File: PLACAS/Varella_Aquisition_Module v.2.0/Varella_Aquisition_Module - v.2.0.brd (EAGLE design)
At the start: 100 x 80 mm, 70 parts, among them IC1 M95M04-DRDW6TP, IC10 ICL7660SCBAZ, IC3 M95M04-DRDW6TP, IC4 M95M04-DRDW6TP, IC9 M95M04-DRDW6TP, U1 FT232RLSSOP, X2 USB-SMD-NS, Y2 FA-20H_16.0000MF10Z-AJ0

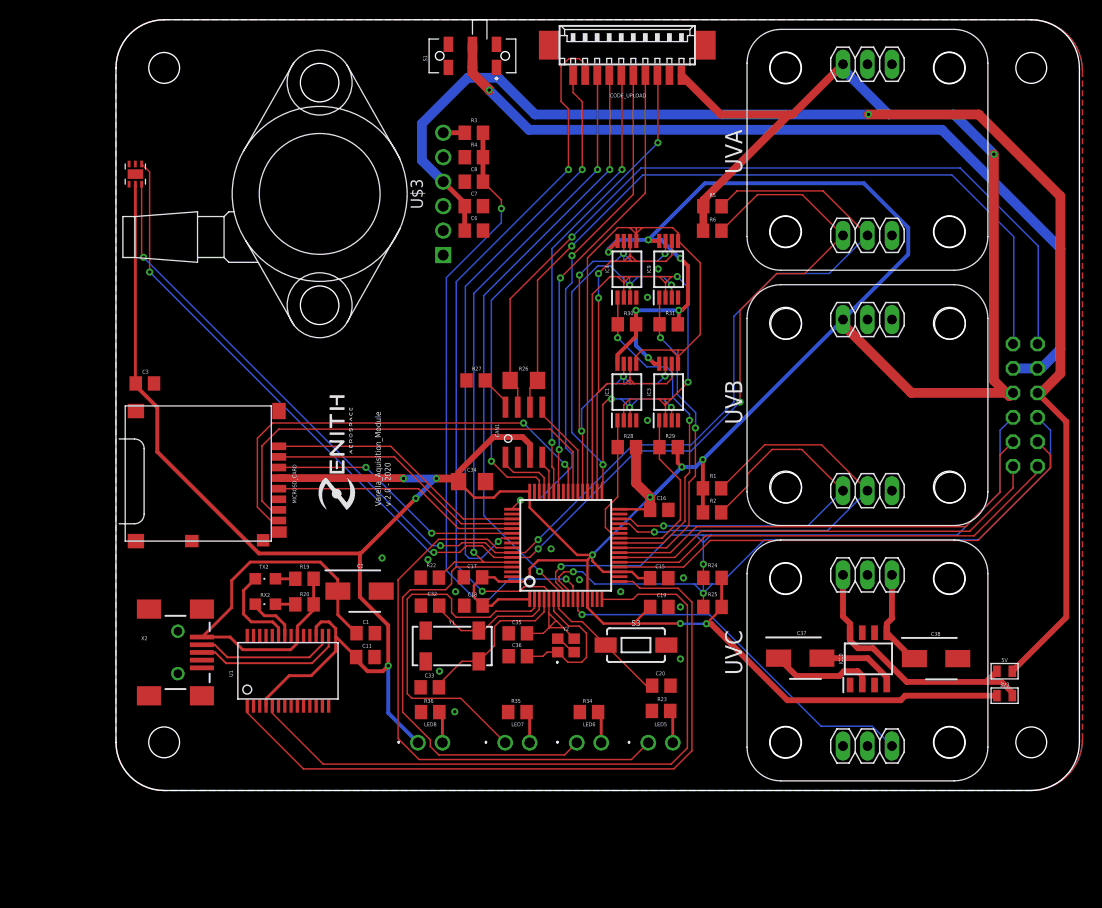
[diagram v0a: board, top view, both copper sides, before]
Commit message: Add files via upload
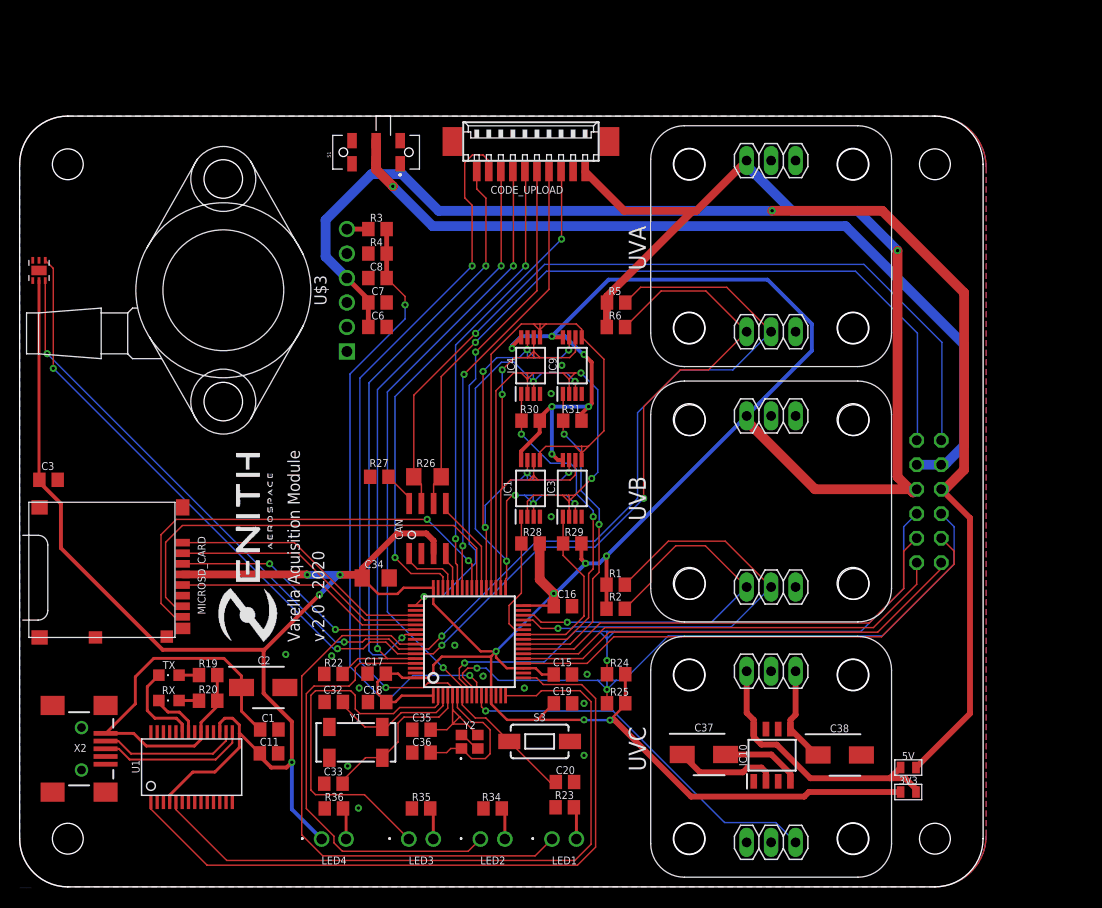
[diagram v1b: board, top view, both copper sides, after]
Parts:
- removed CAN1: SN65HVD233D, SN65HVD233D:SOIC8
- removed LED5, LED6, LED7, LED8: TLLG4400-AS12, SamacSys_Parts:TLLG4400AS12
- removed RX2, TX2: (no value), led:CHIPLED_0805
- added CAN: SN65HVD233D, SN65HVD233D:SOIC8
- added LED1, LED2, LED3, LED4: TLLG4400-AS12, SamacSys_Parts:TLLG4400AS12
- added RX, TX: (no value), led:CHIPLED_0805
- moved C20 14.1 mm to (56.6, 10.9)
- moved COMM_MICRO2 14.1 mm to (46.7, 25.4)
- moved IC3 14.1 mm to (57.4, 41.4)
- moved R29 14.1 mm to (57.4, 35.6)
- moved R6 14.1 mm to (61.9, 58.1)
- moved U$2 14.1 mm to (2.01, 64.0)
- moved U$3 14.1 mm to (34.0, 55.6)
- moved 3V3 14.1 mm to (92.2, 9.84)
- moved 5V 14.1 mm to (92.2, 12.4)
- moved C11 14.1 mm to (25.9, 13.9)
- moved C18 14.1 mm to (37.1, 19.2)
- moved C2 14.1 mm to (25.3, 20.7)
- moved C3 14.1 mm to (3.00, 42.2)
- moved C32 14.1 mm to (32.6, 19.2)
- moved C33 14.1 mm to (32.6, 10.7)
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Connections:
- net +3V3: now also CAN.3, LED4.1; no longer CAN1.3, LED8.1
- net CAN1_LBK: now also CAN.5; no longer CAN1.5
- net CAN1_RX: now also CAN.4; no longer CAN1.4
- net CAN1_TX: now also CAN.1; no longer CAN1.1
- net CAN_H: now also CAN.7; no longer CAN1.7
- net CAN_L: now also CAN.6; no longer CAN1.6
- net GND: now also CAN.2; no longer CAN1.2
- net LED_DEBUG: now also LED3.1; no longer LED7.1
- net LED_SD: now also LED1.1; no longer LED5.1
- net LED_USB: now also LED2.1; no longer LED6.1
- net N$11: now also CAN.8; no longer CAN1.8
- net N$16: now also LED1.2; no longer LED5.2
- net N$17: now also LED2.2; no longer LED6.2
- net N$19: now also LED3.2; no longer LED7.2
- net N$20: now also LED4.2; no longer LED8.2
- net RXL: now also RX.A; no longer RX2.A
- net RXLED: now also RX.C; no longer RX2.C
- net TXL: now also TX.A; no longer TX2.A
- net TXLED: now also TX.C; no longer TX2.C
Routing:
- net +3V3: track 487.9 -> 487.3 mm
- net MISO_MEMORY: track 62.1 -> 62.6 mm
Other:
- board text added: "C:/Users/marcu/Desktop/zenith-v3.bmp"
- board text added: "Varella Aquisition Module"
- board text removed: "Varella_Aquisition_Module"
